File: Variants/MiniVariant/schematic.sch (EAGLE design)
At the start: 12 parts, among them U1 TMP75_D_8, U2 SHT21

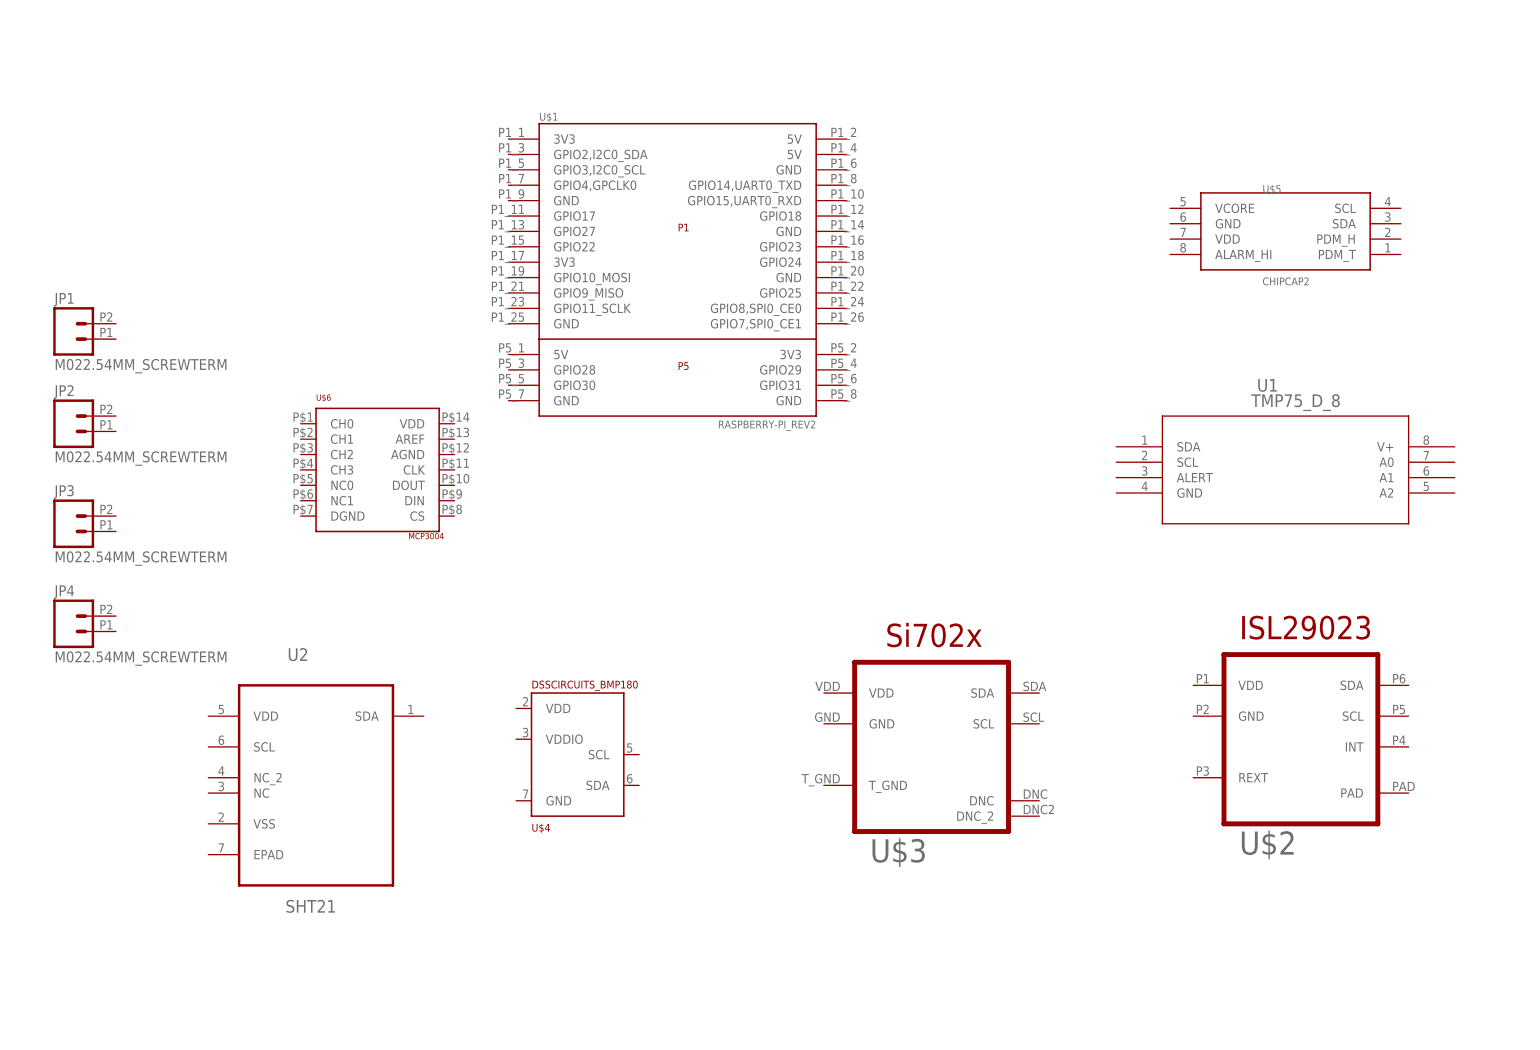
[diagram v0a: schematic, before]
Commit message: Normal Push
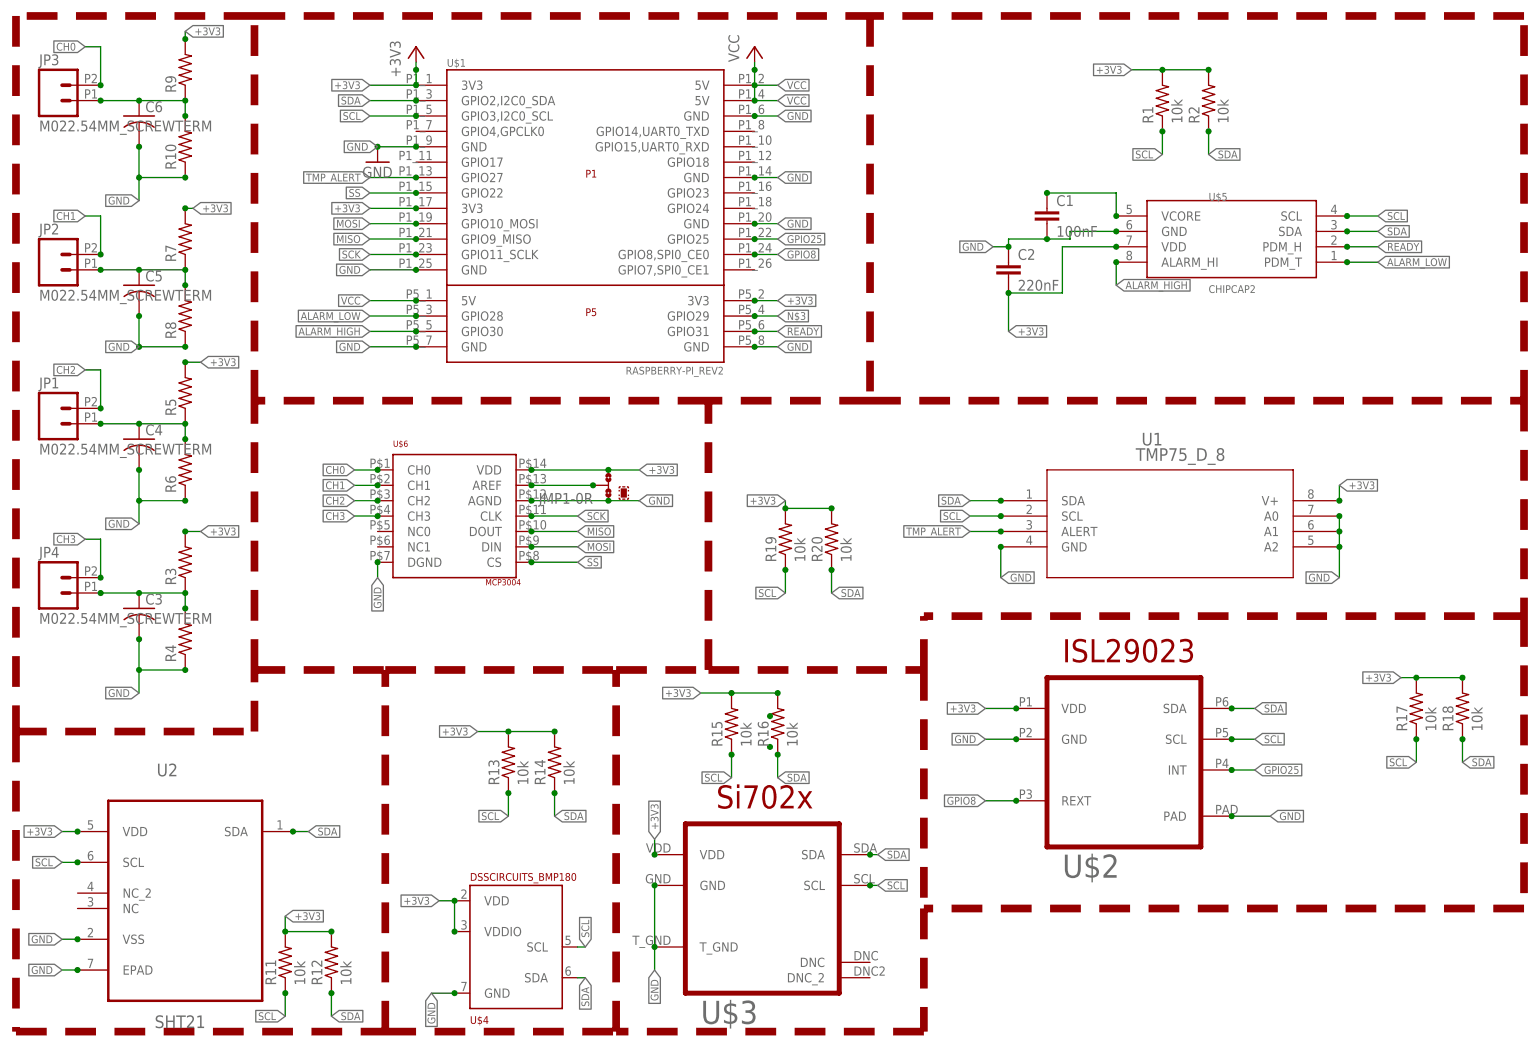
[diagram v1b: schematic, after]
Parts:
- added C1: 100nF, weatherpilot_lbr:CAP0402-CAP
- added C2: 220nF, weatherpilot_lbr:CAP0402-CAP
- added C3, C4, C5, C6: (no value), rcl:C-USC0402
- added JMP1: 0R-JUMPA, jump-0r-smd:0R-JUMPA
- added R1, R11, R12, R13, R14, R15, R16, R17, R18, R19, R2, R20: 10k, SparkFun-Resistors:RESISTOR0603
- added R10, R3, R4, R5, R6, R7, R8, R9: (no value), rcl:R-US_R0402
- U$1: device lib:RASPBERRY-PI_REV2 -> RaspberryPi:RASPBERRY-PI_REV2
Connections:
- new net +3V3: C2.2, JMP1-0R.3, R1.2, R11.2, R12.2, R13.2, R14.2, R15.2, R16.2, R17.2, R18.2, R19.2, R2.2, R20.2, R3.2, R5.2, R7.2, R9.2, U$1.3V3@1, U$1.3V3@17, U$1.3V3@P5_2, U$2.VDD, U$3.VDD, U$4.VDD, U$4.VDDIO, U$5.VDD, U$6.VDD, U1.V+, U2.VDD
- new net ALARM_HIGH: U$1.GPIO30, U$5.ALARM_HI
- new net ALARM_LOW: U$1.GPIO28, U$5.PDM_T
- new net CH0: JP3.2, U$6.CH0
- new net CH1: JP2.2, U$6.CH1
- new net CH2: JP1.2, U$6.CH2
- new net CH3: JP4.2, U$6.CH3
- new net GND: C1.2, C2.1, C3.2, C4.2, C5.2, C6.2, JMP1-0R.1, R10.1, R4.1, R6.1, R8.1, U$1.GND@14, U$1.GND@20, U$1.GND@25, U$1.GND@6, U$1.GND@9, U$1.GND@P5_7, U$1.GND@P5_8, U$2.GND, U$2.PAD, U$3.GND, U$3.T_GND, U$4.GND, U$5.GND, U$6.AGND, U$6.DGND, U1.A0, U1.A1, U1.A2, U1.GND, U2.EPAD, U2.VSS
- new net GPIO25: U$1.GPIO25, U$2.INT
- new net GPIO8: U$1.GPIO8,SPI0_CE0, U$2.REXT
- new net MISO: U$1.GPIO9_MISO, U$6.DOUT
- new net MOSI: U$1.GPIO10_MOSI, U$6.DIN
- new net N$1: C4.1, JP1.1, R5.1, R6.2
- new net N$12: C3.1, JP4.1, R3.1, R4.2
- new net N$17: JMP1-0R.2, U$6.AREF
- new net N$2: C5.1, JP2.1, R7.1, R8.2
- new net N$3: U$1.GPIO29
- new net N$4: C6.1, JP3.1, R10.2, R9.1
- new net N$5: C1.1, U$5.VCORE
- new net READY: U$1.GPIO31, U$5.PDM_H
- new net SCK: U$1.GPIO11_SCLK, U$6.CLK
- new net SCL: R1.1, R11.1, R13.1, R15.1, R17.1, R19.1, U$1.GPIO3,I2C0_SCL, U$2.SCL, U$3.SCL, U$4.SCL, U$5.SCL, U1.SCL, U2.SCL
- new net SDA: R12.1, R14.1, R16.1, R18.1, R2.1, R20.1, U$1.GPIO2,I2C0_SDA, U$2.SDA, U$3.SDA, U$4.SDA, U$5.SDA, U1.SDA, U2.SDA
- new net SS: U$1.GPIO22, U$6.CS
- new net TMP_ALERT: U$1.GPIO27, U1.ALERT
- new net VCC: U$1.5V@2, U$1.5V@4, U$1.5V@P5_1
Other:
- moved on the sheet: JP1, JP2, JP3, JP4, U$1, U$2, U$3, U$4, U$5, U$6, U1, U2
